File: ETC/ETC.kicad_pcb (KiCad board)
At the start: 2 copper layers, 96.5 x 100.5 mm, 36 parts, among them P1 DTM1312PC12PDR008, U1 NUCLEO-F446RE, U2 MCP6004, U3 LM7805_TO220, U4 LM7809_TO220, U5 ISO1050DUB, U6 ISO1050DUB, U7 SN74AHC14N

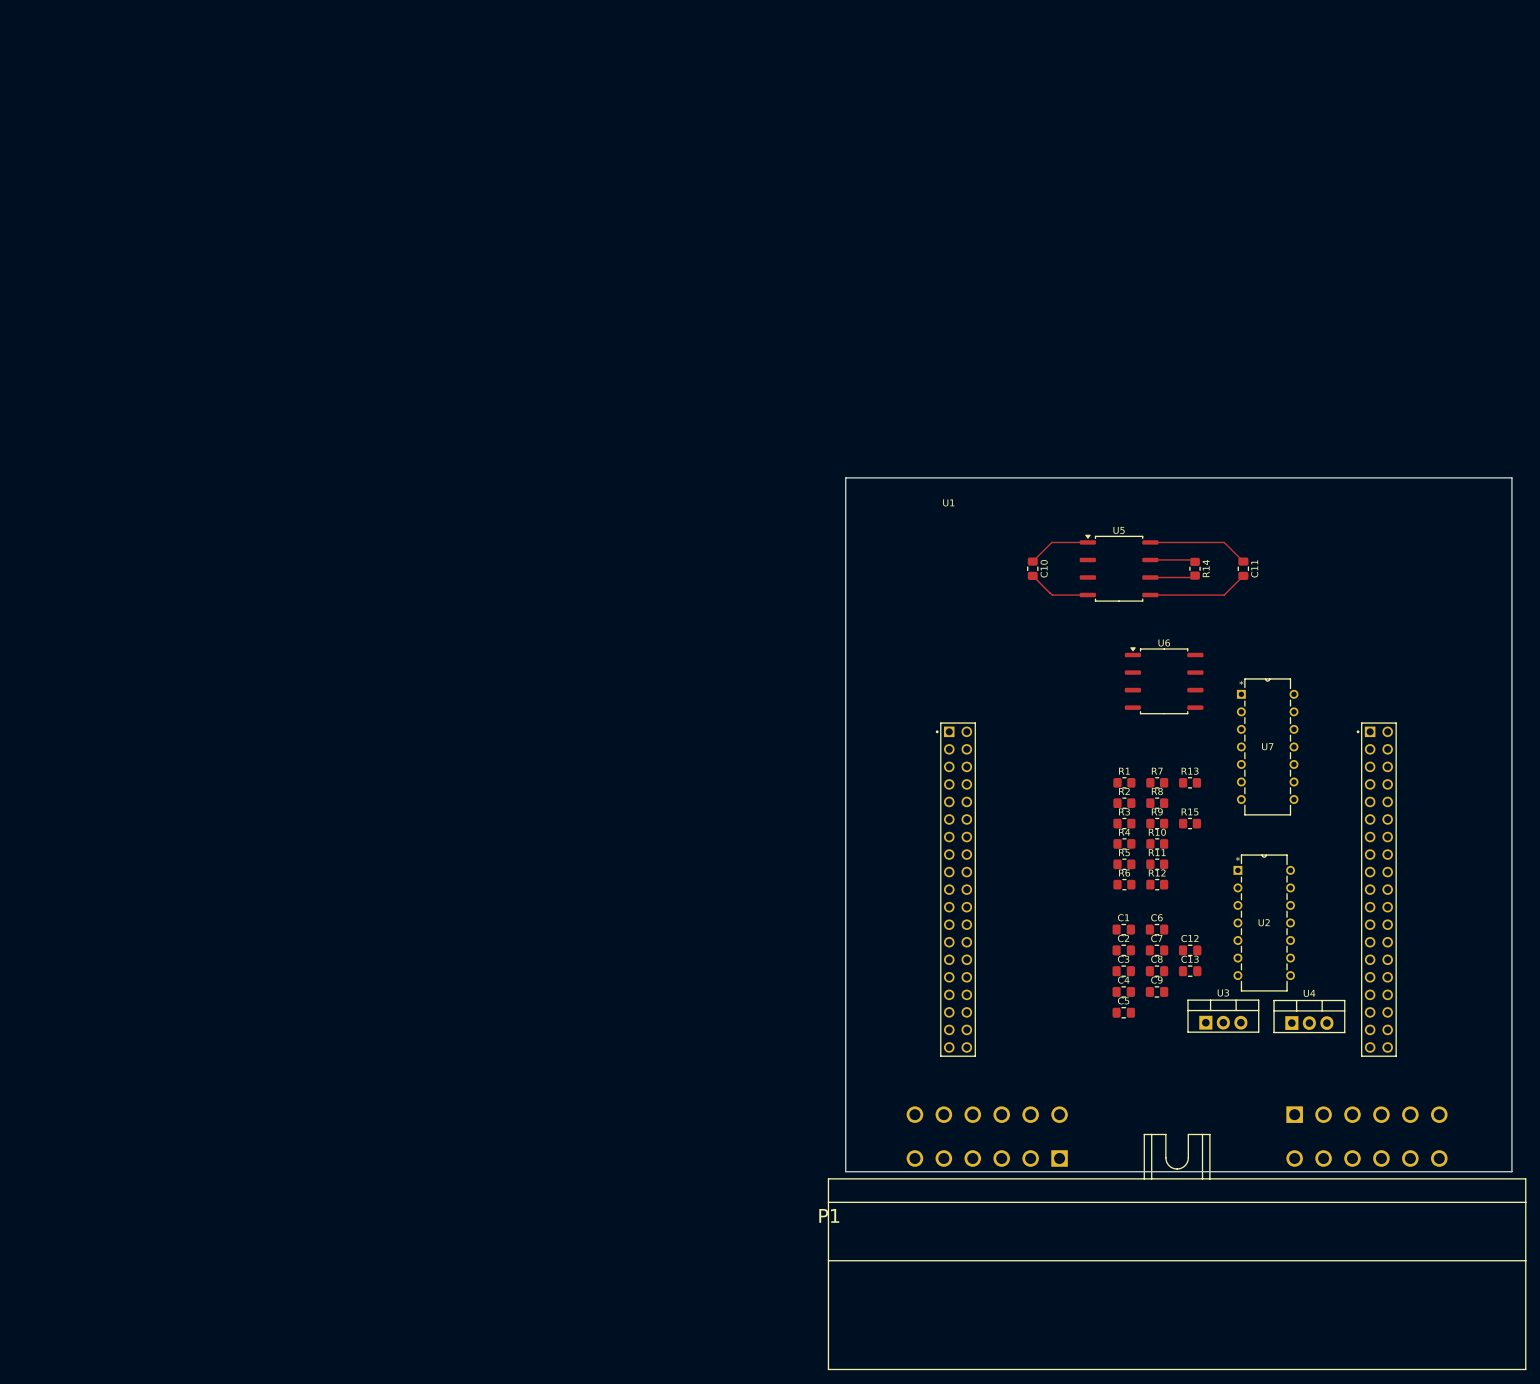
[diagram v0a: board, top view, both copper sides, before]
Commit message: working directory
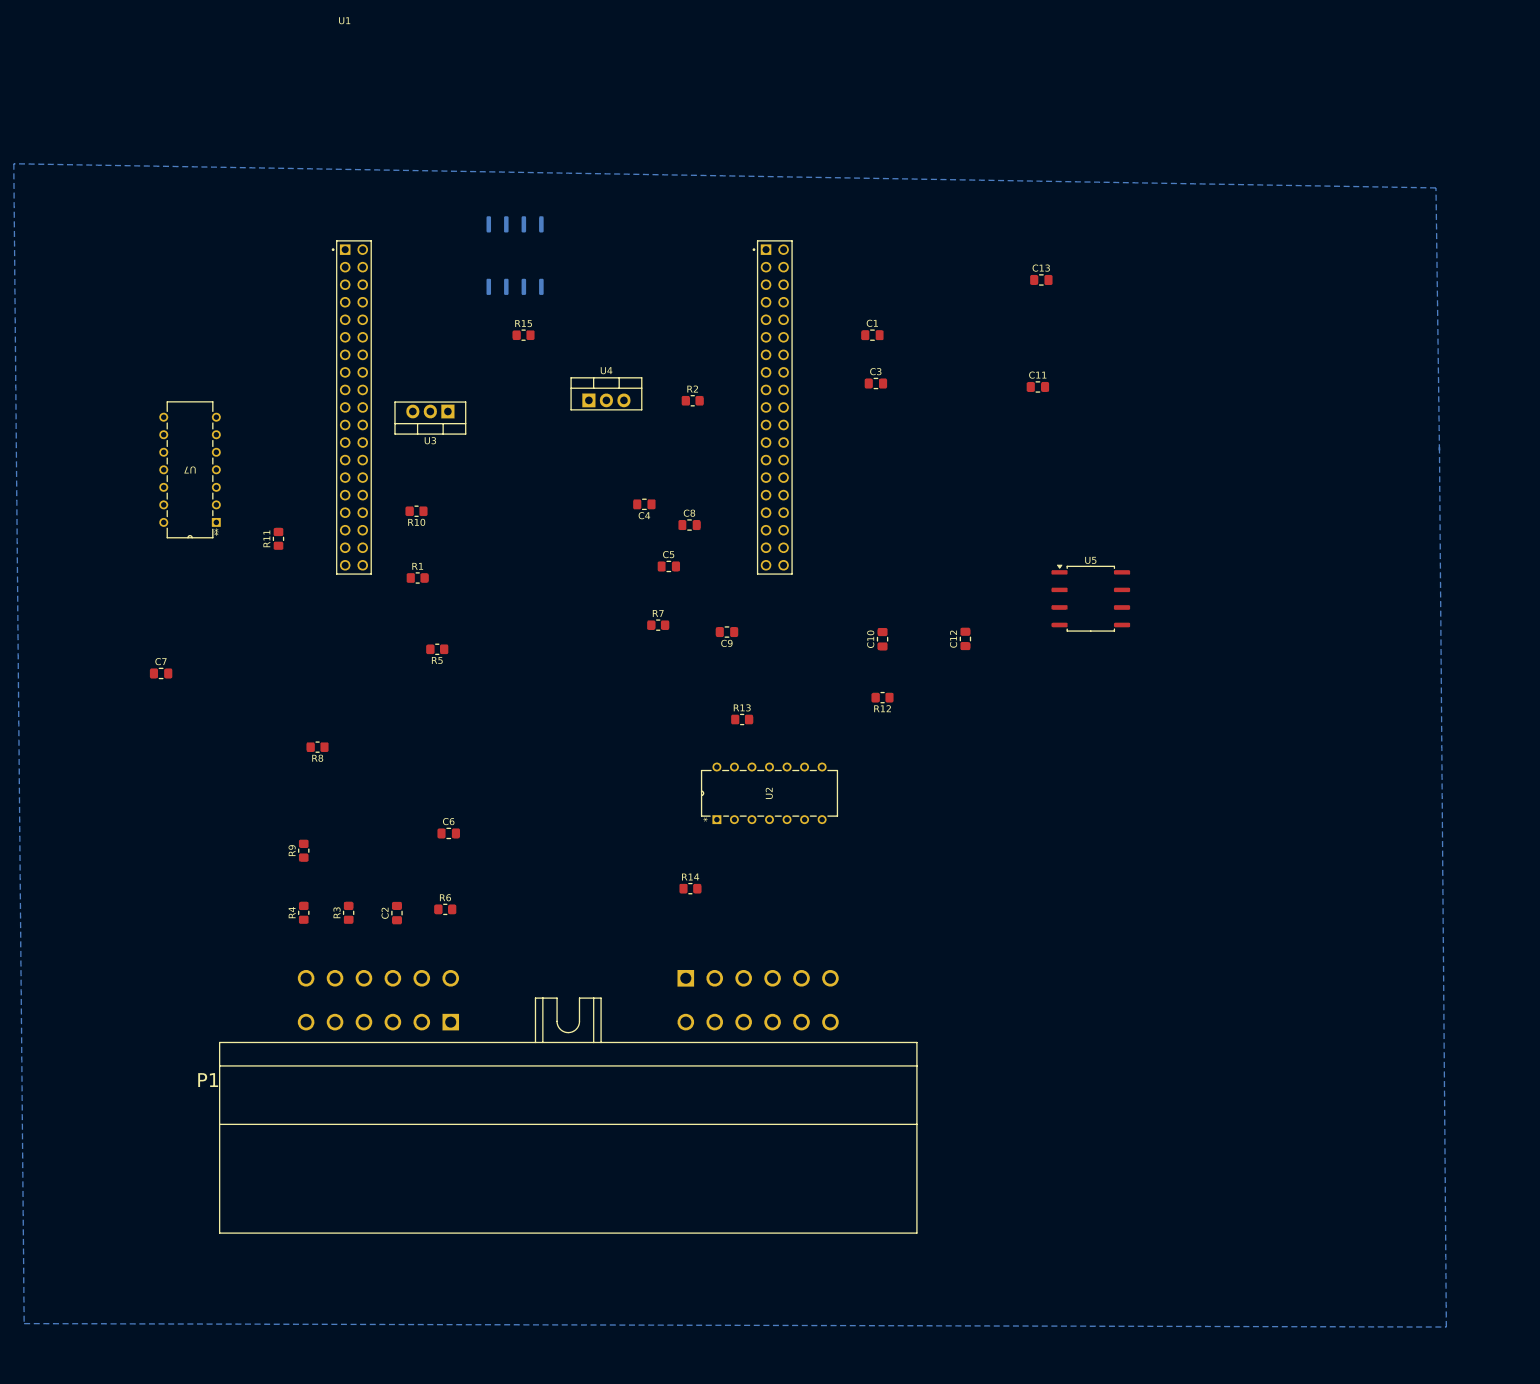
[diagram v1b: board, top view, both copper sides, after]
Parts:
- U6: moved to B.Cu
- moved U7 172.8 mm to (52.2, 52.7), turned to 180 degrees
- moved C7 149.7 mm to (51.8, 89.8)
- moved U3 141.0 mm to (93.4, 51.9), turned to 180 degrees
- moved U4 136.0 mm to (113.8, 50.3)
- moved R11 135.7 mm to (68.8, 70.3), turned to 90 degrees
- moved R9 123.7 mm to (72.5, 115.5), turned to 90 degrees
- moved R8 121.9 mm to (74.5, 100.5), turned to 180 degrees
- moved R15 119.7 mm to (104.3, 40.8)
- moved R4 119.3 mm to (72.5, 124.5), turned to 90 degrees
- moved R10 117.6 mm to (88.8, 66.3), turned to 180 degrees
- moved R3 113.1 mm to (79.0, 124.5), turned to 90 degrees
- moved U6 112.4 mm to (103.1, 29.3), turned to -90 degrees
- moved U1 112.0 mm to (110.2, 38.0)
- moved R1 106.6 mm to (89.0, 76.0)
- moved C2 105.4 mm to (86.0, 124.5), turned to 90 degrees
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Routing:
- net GND: track 23.7 -> 0.00 mm
- net +5V: track 14.6 -> 0.00 mm
- net +3V3: track 9.12 -> 0.00 mm
- net /L_Motor_CAN: track 6.59 -> 0.00 mm
- net /H_Motor_CAN: track 6.59 -> 0.00 mm
- added copper zone on B.Cu, net GND
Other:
- board outline removed
